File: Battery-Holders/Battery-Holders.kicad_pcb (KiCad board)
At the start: 2 copper layers, 92.7 x 142.2 mm, 12 parts, among them J1 Conn_01x02

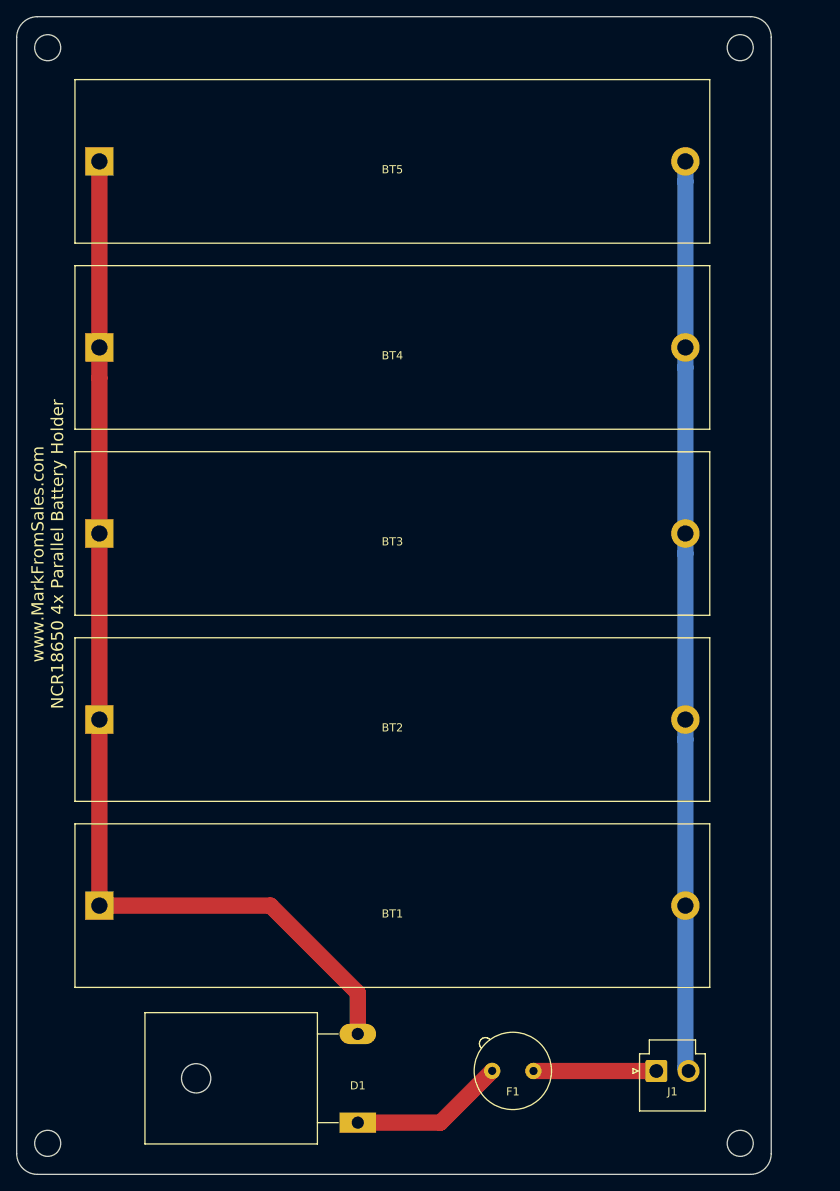
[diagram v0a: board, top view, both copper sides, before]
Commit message: minor
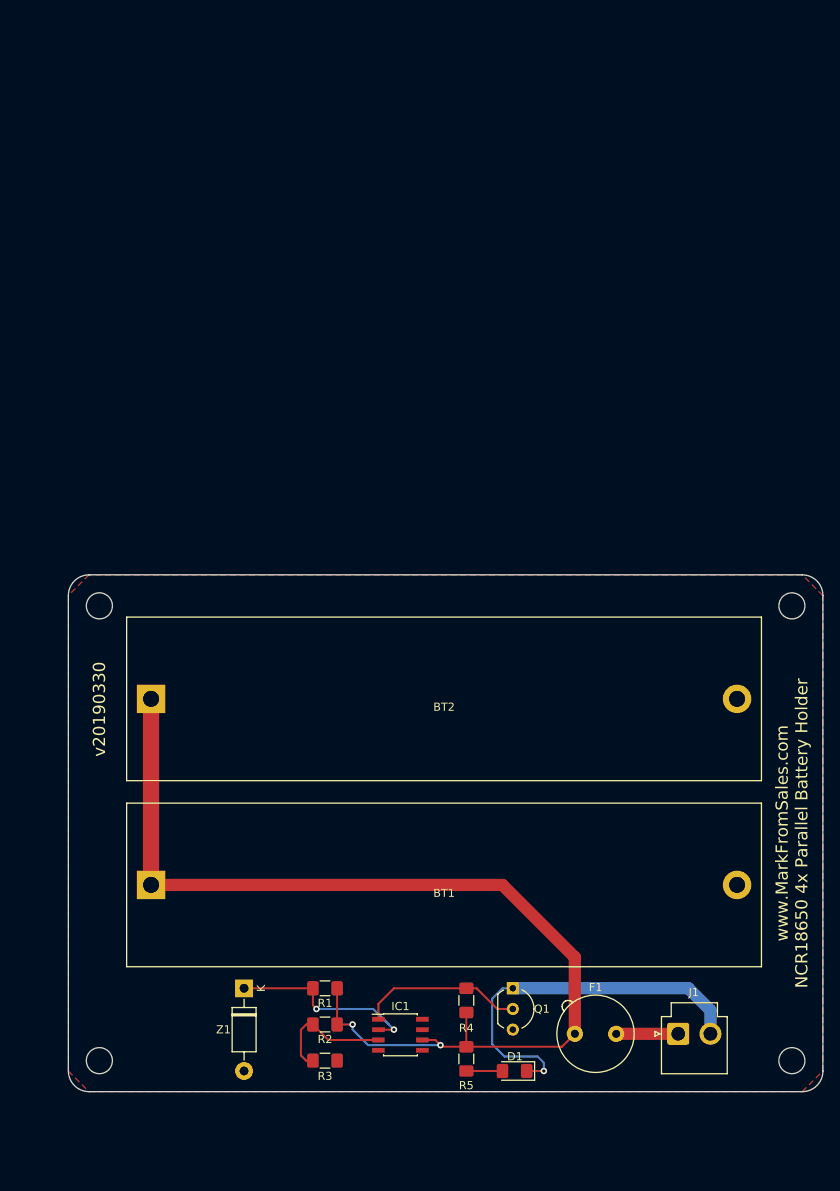
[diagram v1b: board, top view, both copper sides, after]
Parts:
- removed BT3, BT4, BT5: Battery, Battery:BatteryHolder_MPD_BH-18650-PC2
- added IC1: LM393DR, Package_SO:SOIC-8_3.9x4.9mm_P1.27mm, F.Cu at (87.8, 158.1)
- added Q1: BS170, Package_TO_SOT_THT:TO-92_Inline_Wide, F.Cu at (101.6, 152.4)
- added R1: R, Resistor_SMD:R_1206_3216Metric_Pad1.42x1.75mm_HandSolder, F.Cu at (78.5, 152.4)
- added R2: R, Resistor_SMD:R_1206_3216Metric_Pad1.42x1.75mm_HandSolder, F.Cu at (78.5, 156.8)
- added R3: R, Resistor_SMD:R_1206_3216Metric_Pad1.42x1.75mm_HandSolder, F.Cu at (78.5, 161.3)
- added R4: R, Resistor_SMD:R_1206_3216Metric_Pad1.42x1.75mm_HandSolder, F.Cu at (95.9, 153.9)
- added R5: R, Resistor_SMD:R_1206_3216Metric_Pad1.42x1.75mm_HandSolder, F.Cu at (95.9, 161.1)
- added Z1: 1N4733A, Diode_THT:D_DO-41_SOD81_P10.16mm_Horizontal, F.Cu at (68.6, 152.4)
- D1: value D -> LED; footprint Package_TO_SOT_THT:TO-247-2_Horizontal_TabDown -> LED_SMD:LED_1206_3216Metric_Pad1.42x1.75mm_HandSolder
- moved H1 68.9 mm to (50.8, 105.4)
- moved H2 68.9 mm to (135.9, 105.4)
- moved D1 20.3 mm to (101.8, 162.6), turned to 180 degrees
- moved H3 12.0 mm to (50.8, 161.3)
- moved H4 12.0 mm to (135.9, 161.3)
- moved F1 11.1 mm to (114.3, 158.0)
- moved BT1 6.84 mm to (57.1, 139.7)
- moved BT2 6.84 mm to (57.1, 116.8)
- moved J1 5.30 mm to (121.9, 158.0)
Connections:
- BT1 pad 2: Net-(BT1-Pad2) -> GND
- BT2 pad 2: Net-(BT1-Pad2) -> GND
- D1 pad 2: Net-(BT1-Pad1) -> Net-(D1-Pad2)
- F1 pad 2: Net-(D1-Pad1) -> Net-(BT1-Pad1)
- J1 pad 2: Net-(BT1-Pad2) -> Net-(D1-Pad1)
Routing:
- net Net-(BT1-Pad2): track 111.9 -> 0.00 mm
- net Net-(D1-Pad1): track 19.1 -> 47.4 mm, vias 0 -> 1
- net Net-(IC1-Pad2): track 0.00 -> 25.5 mm, vias 0 -> 2
- net Net-(IC1-Pad1): track 0.00 -> 20.3 mm
- net Net-(IC1-Pad3): track 0.00 -> 15.5 mm
- net Net-(F1-Pad1): track 15.1 -> 7.62 mm
- net Net-(D1-Pad2): track 0.00 -> 4.44 mm
- net Net-(BT1-Pad1): track 132.7 -> 130.5 mm, vias 0 -> 2
- added copper zone on F.Cu, net GND
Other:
- board size 92.7 x 142.2 mm -> 92.7 x 63.5 mm
- board text added: "v20190330"
